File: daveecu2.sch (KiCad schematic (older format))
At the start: 6 parts, among them J1 CONN_BLACK, J2 CONN_GREY

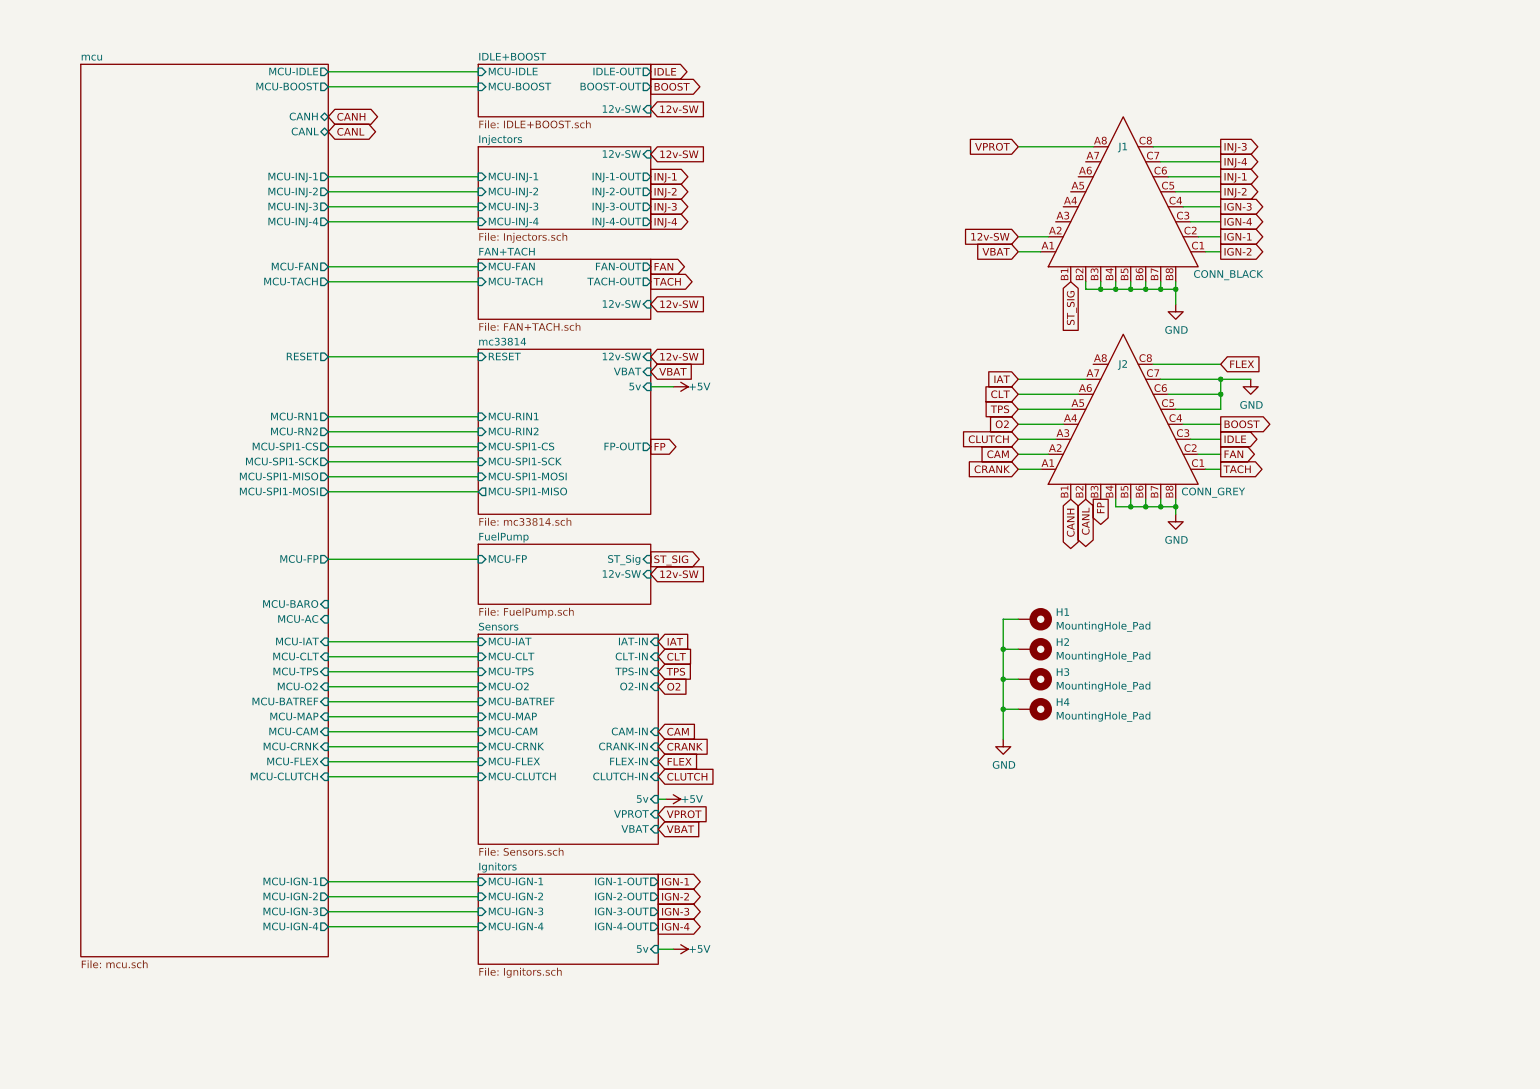
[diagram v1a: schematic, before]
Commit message: Update Schematic with a bunch of extra stuff
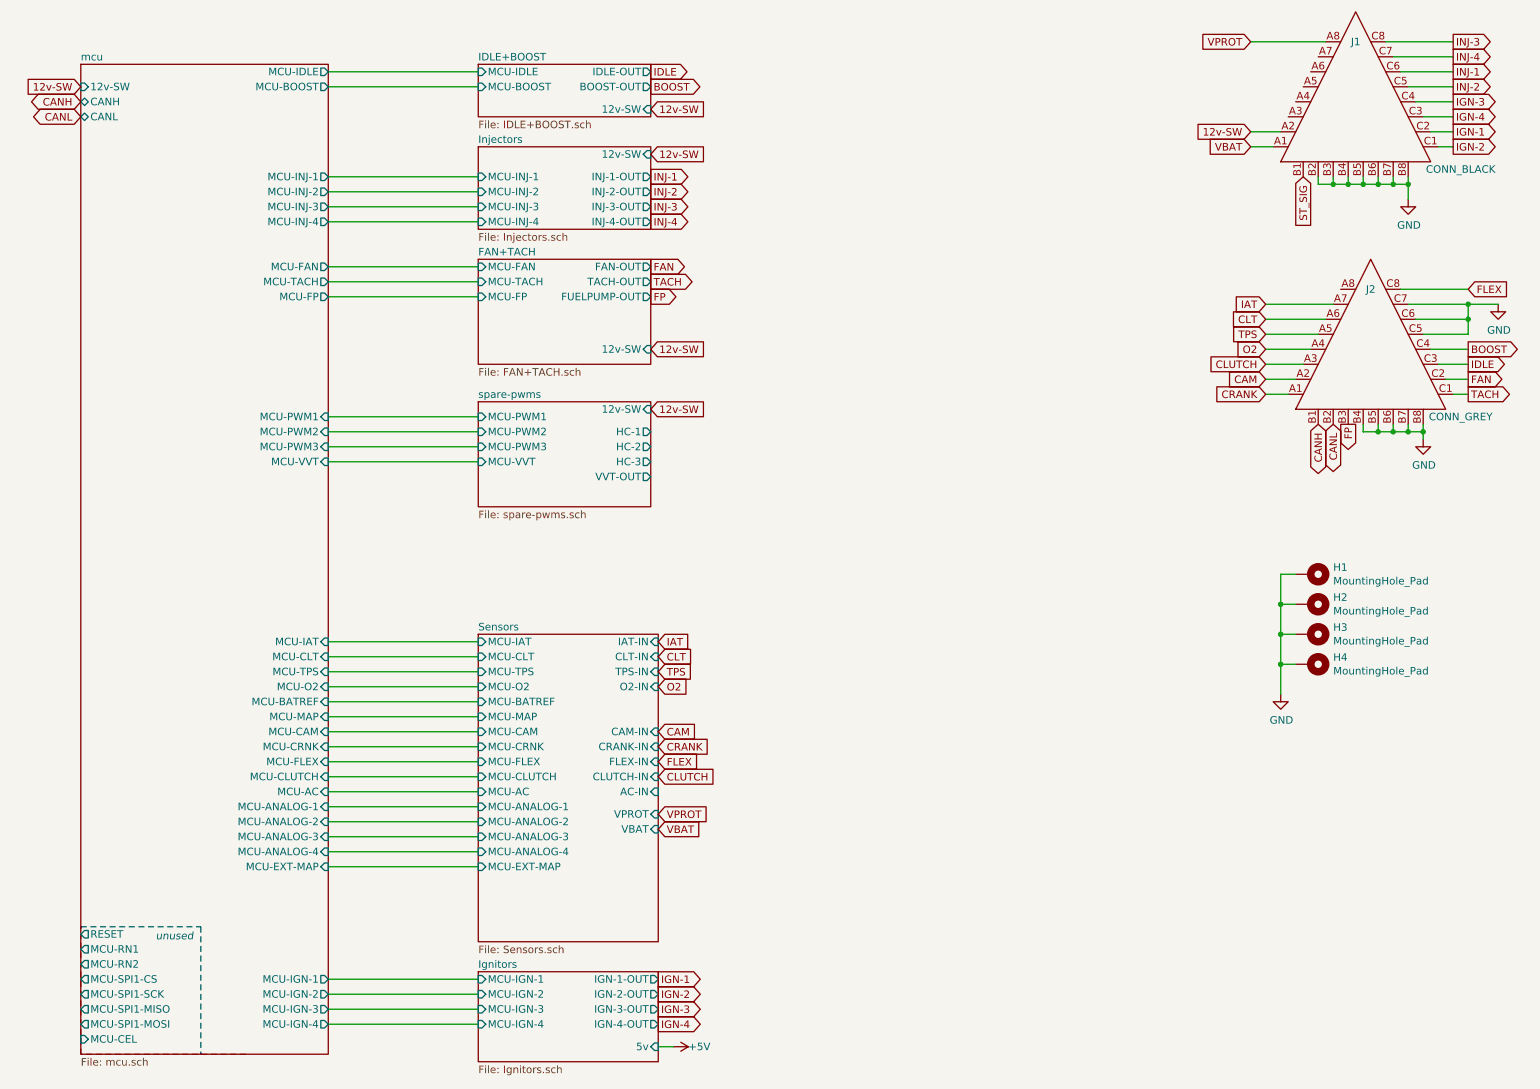
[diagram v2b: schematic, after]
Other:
- note added: "unused"
- moved on the sheet: H1, H2, H3, H4, J1, J2

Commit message: Finish reroute again
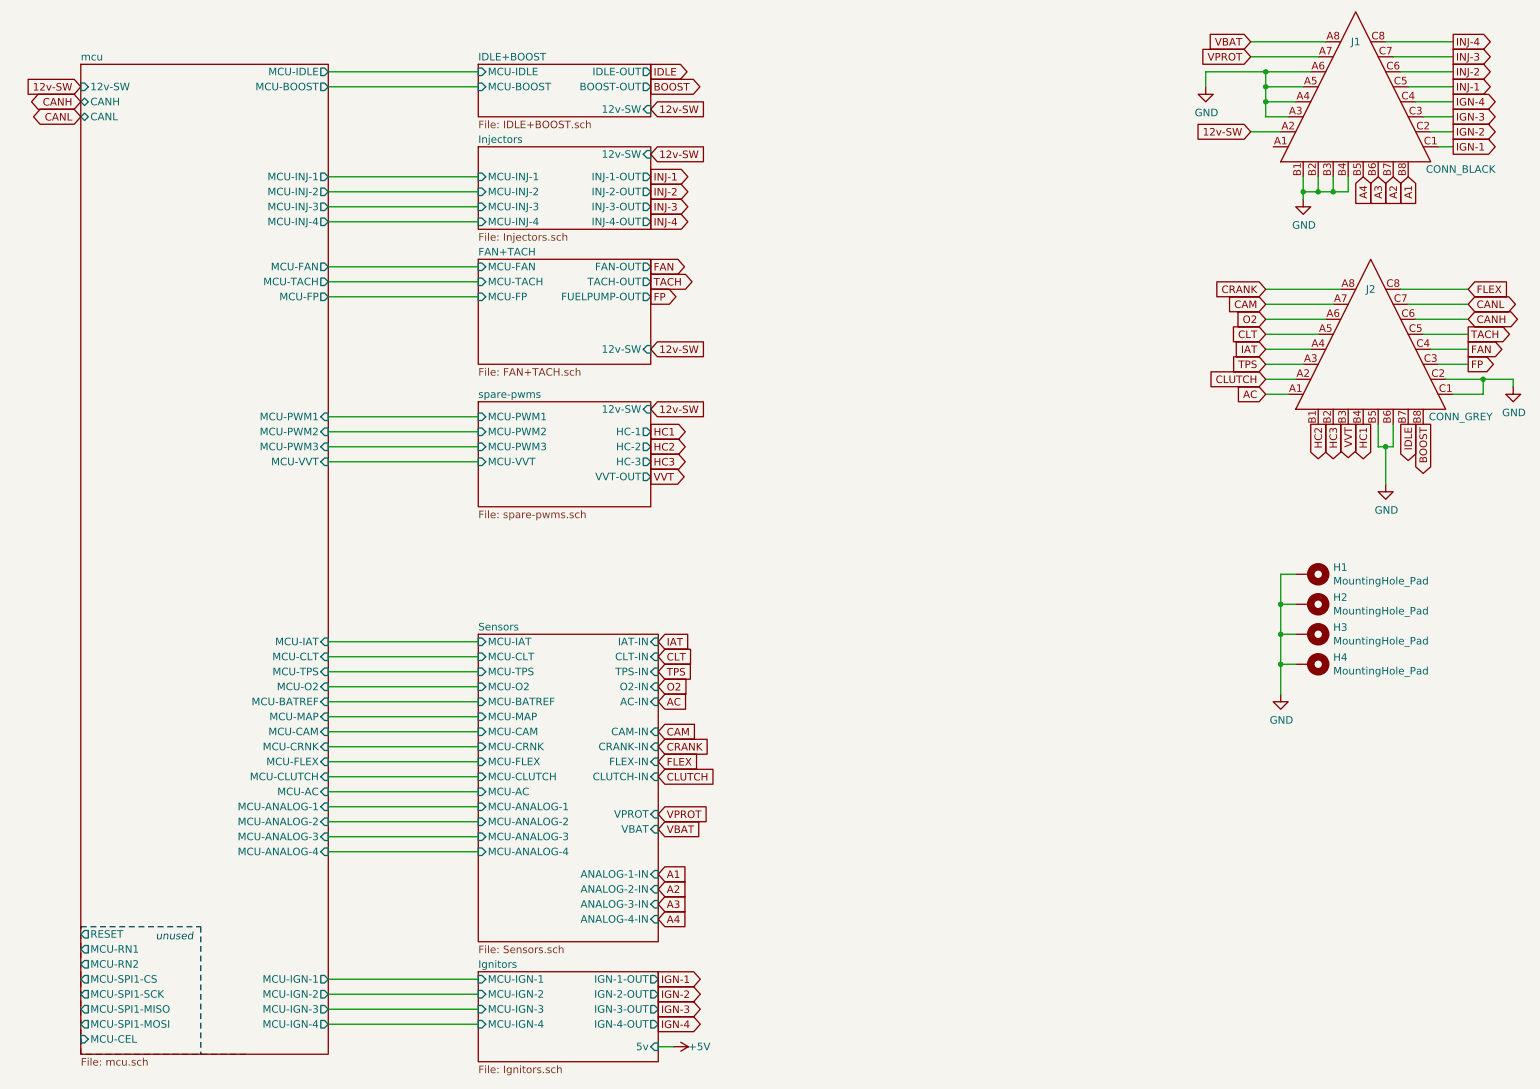
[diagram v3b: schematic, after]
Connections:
- net ST_SIG is gone; now on net GND: J1.B1
- net BOOST: now also J2.B8; no longer J2.C4
- net CAM: now also J2.A7; no longer J2.A2
- net CANH: now also J2.C6; no longer J2.B1
- net CANL: now also J2.C7; no longer J2.B2
- net CLT: now also J2.A5; no longer J2.A6
- net CLUTCH: now also J2.A2; no longer J2.A3
- net CRANK: now also J2.A8; no longer J2.A1
- net FAN: now also J2.C4; no longer J2.C2
- net FP: now also J2.C3; no longer J2.B3
- net GND: now also J1.A3, J1.A4, J1.A5, J1.A6, J2.C1, J2.C2; no longer J1.B5, J1.B6, J1.B7, J1.B8, J2.B4, J2.B7, J2.B8, J2.C5, J2.C6, J2.C7
- net IAT: now also J2.A4; no longer J2.A7
- net IDLE: now also J2.B7; no longer J2.C3
- net IGN-1: now also J1.C1; no longer J1.C2
- net IGN-2: now also J1.C2; no longer J1.C1
- net IGN-3: now also J1.C3; no longer J1.C4
- net IGN-4: now also J1.C4; no longer J1.C3
- net INJ-1: now also J1.C5; no longer J1.C6
- net INJ-2: now also J1.C6; no longer J1.C5
- net INJ-3: now also J1.C7; no longer J1.C8
- net INJ-4: now also J1.C8; no longer J1.C7
- net O2: now also J2.A6; no longer J2.A4
- net TACH: now also J2.C5; no longer J2.C1
- net TPS: now also J2.A3; no longer J2.A5
- net VBAT: now also J1.A8; no longer J1.A1
- net VPROT: now also J1.A7; no longer J1.A8
- new net A1: J1.B8
- new net A2: J1.B7
- new net A3: J1.B6
- new net A4: J1.B5
- new net AC: J2.A1
- new net HC1: J2.B4
- new net HC2: J2.B1
- new net HC3: J2.B2
- new net VVT: J2.B3
